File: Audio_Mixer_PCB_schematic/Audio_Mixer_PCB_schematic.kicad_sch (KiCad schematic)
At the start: 70 parts, among them U1 Avol=1Meg GBW=10Meg Vos=0, U11 Avol=1Meg GBW=10Meg Vos=0, U12 Avol=1Meg GBW=10Meg Vos=0, U13 Avol=1Meg GBW=10Meg Vos=0, U14 Avol=1Meg GBW=10Meg Vos=0, U15 Avol=1Meg GBW=10Meg Vos=0, U16 Avol=1Meg GBW=10Meg Vos=0, U17 Avol=1Meg GBW=10Meg Vos=0, U2 Avol=1Meg GBW=10Meg Vos=0, U3 Avol=1Meg GBW=10Meg Vos=0, U4 Avol=1Meg GBW=10Meg Vos=0, U5 Avol=1Meg GBW=10Meg Vos=0, U6 Avol=1Meg GBW=10Meg Vos=0

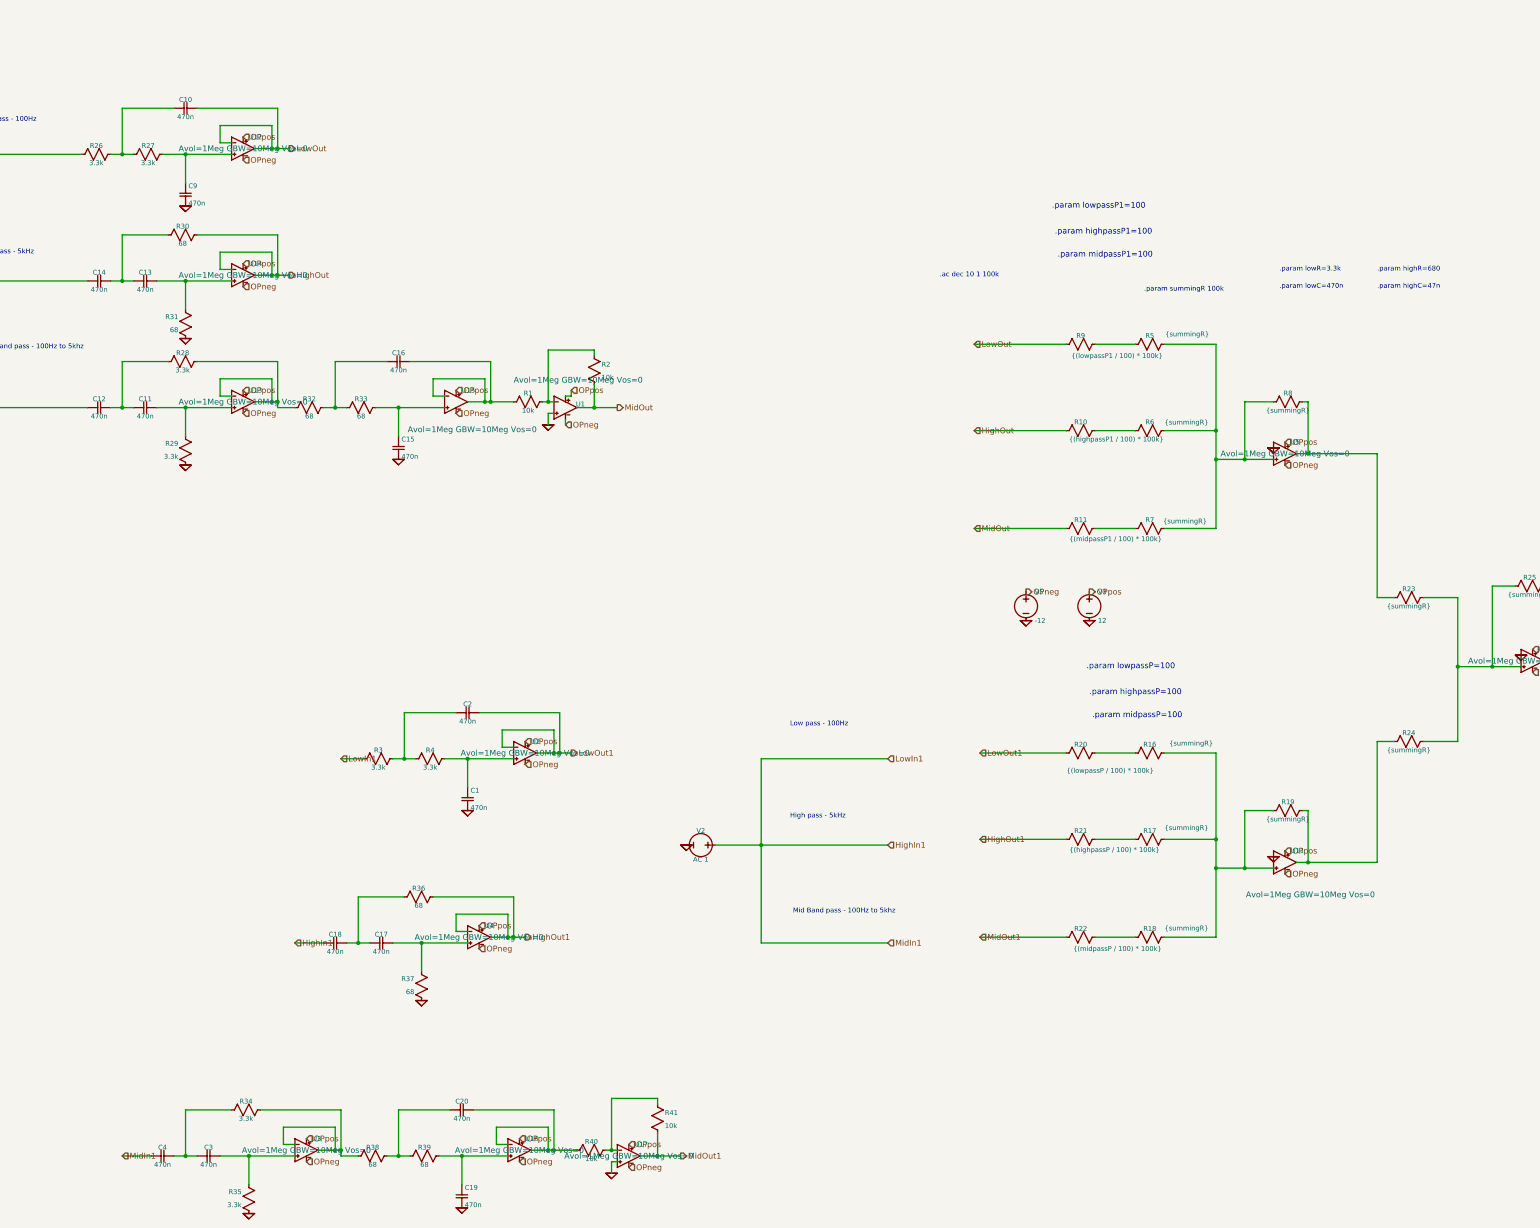
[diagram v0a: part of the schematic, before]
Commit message: more sch stuff
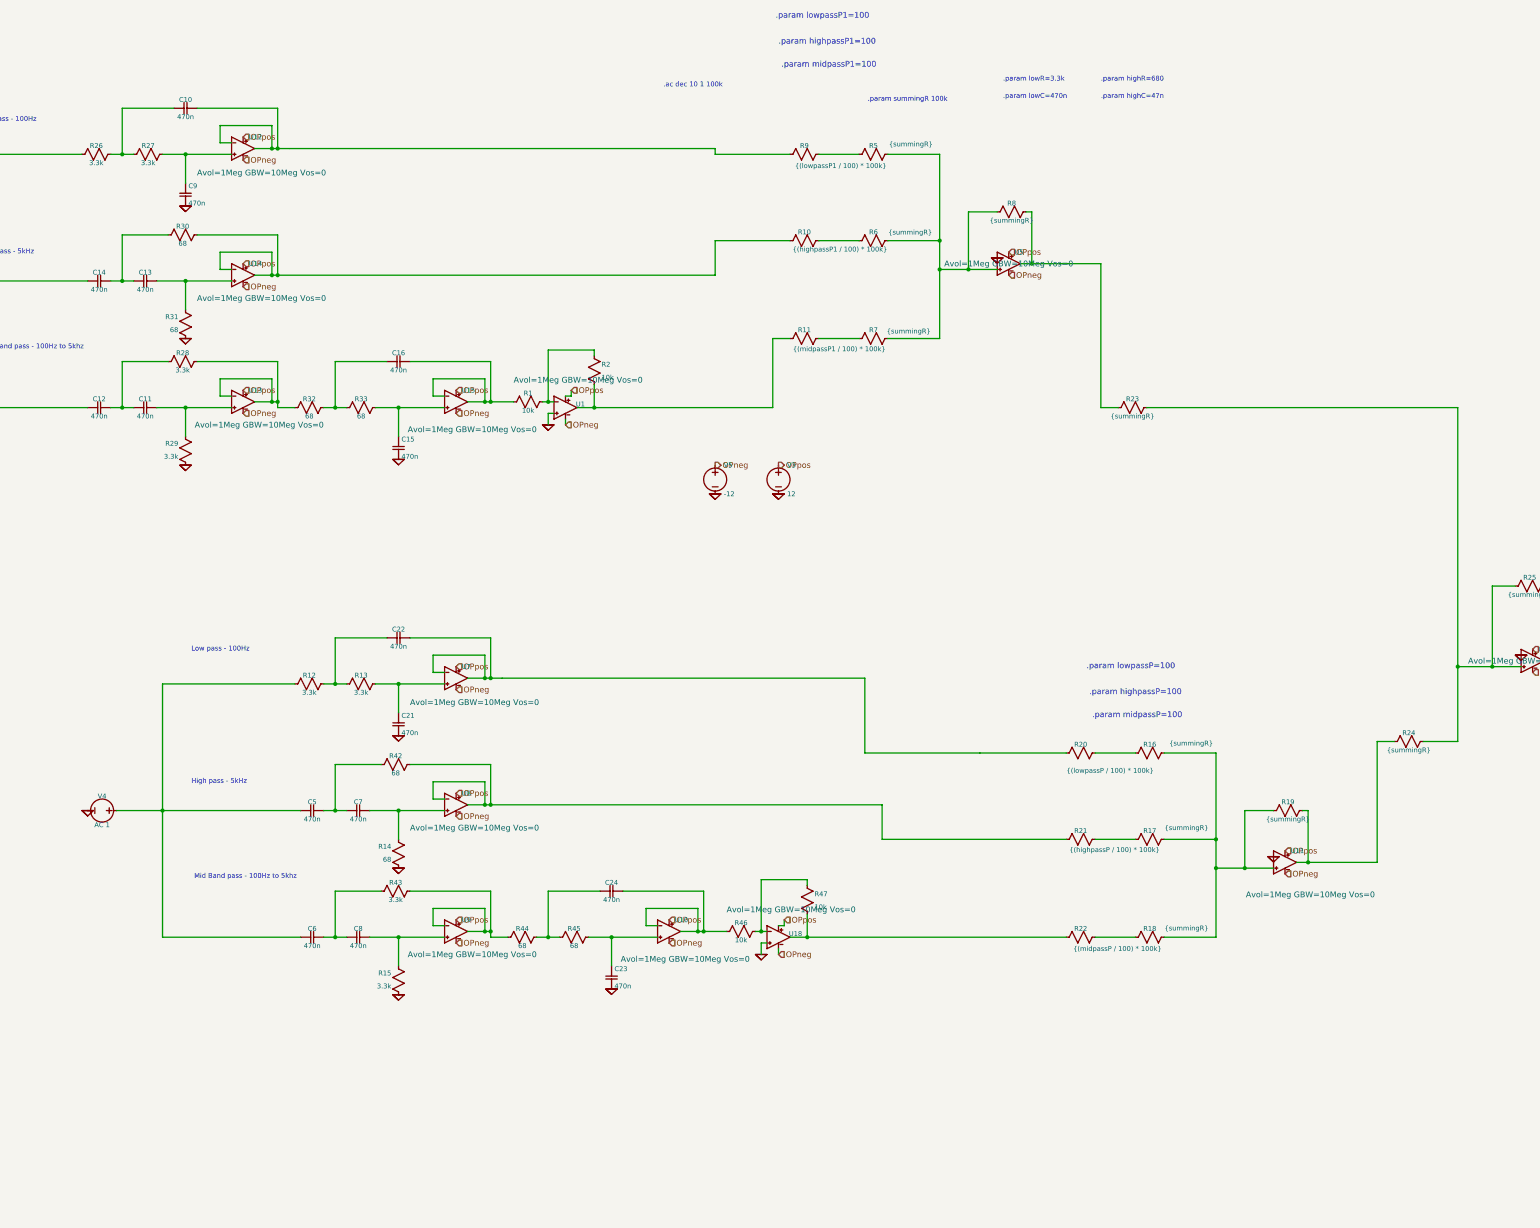
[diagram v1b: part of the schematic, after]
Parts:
- removed C1, C17, C18, C19, C2, C20, C3, C4: 470n, symbol ltspice:cap
- removed R3, R34, R35, R4: 3.3k, symbol ltspice:res
- removed R36, R37, R38, R39: 68, symbol ltspice:res
- removed R40, R41: 10k, symbol ltspice:res
- removed U16, U17, U2, U3, U4: Avol=1Meg GBW=10Meg Vos=0, symbol ltspice:OpAmps/UniversalOpAmp
- removed V2: AC 1, symbol ltspice:Voltage
- added C21, C22, C23, C24, C5, C6, C7, C8: 470n, symbol ltspice:cap
- added R12, R13, R15, R43: 3.3k, symbol ltspice:res
- added R14, R42, R44, R45: 68, symbol ltspice:res
- added R46, R47: 10k, symbol ltspice:res
- added U10, U18, U7, U8, U9: Avol=1Meg GBW=10Meg Vos=0, symbol ltspice:OpAmps/UniversalOpAmp
- added V4: AC 1, symbol ltspice:Voltage
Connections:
- net 0: now also C21.2, C23.2, R14.1, R15.1, U18.1 (In+), V4.2 (-)
- net OPneg: now also U10.4 (V-), U18.4 (V-), U7.4 (V-), U8.4 (V-), U9.4 (V-)
- net OPpos: now also U10.3 (V+), U18.3 (V+), U7.3 (V+), U8.3 (V+), U9.3 (V+)
- net HighOut: no longer names the net of R10.2, R30.1, U14.2 (In-), U14.5 (OUT)
- net HighOut1: no longer names the net of R21.2
- net HighOut1: now also R42.1, U8.2 (In-), U8.5 (OUT)
- net LowOut: no longer names the net of C10.1, R9.2, U12.2 (In-), U12.5 (OUT)
- net LowOut1: no longer names the net of R20.2
- net LowOut1: now also C22.1, U7.2 (In-), U7.5 (OUT)
- net MidOut: no longer names the net of R11.2, R2.2, U1.5 (OUT)
- net MidOut1: no longer names the net of R22.2
- net MidOut1: now also R47.2, U18.5 (OUT)
- new net: C5.1, C7.2, R42.2
- new net: C5.2, C6.2, R12.2, V4.1 (+)
- new net: C23.1, R45.1, U10.1 (In+)
- new net: C24.2, R44.1, R45.2
- new net: C7.1, R14.2, U8.1 (In+)
- new net: C21.1, R13.1, U7.1 (In+)
- new net: C22.2, R12.1, R13.2
- new net: C8.1, R15.2, U9.1 (In+)
- new net: R46.1, R47.1, U18.2 (In-)
- new net: C24.1, R46.2, U10.2 (In-), U10.5 (OUT)
- new net: R43.1, R44.2, U9.2 (In-), U9.5 (OUT)
- new net: C6.1, C8.2, R43.2
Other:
- moved on the sheet: R10, R11, R23, R5, R6, R7, R8, R9, U5, V3, V5
